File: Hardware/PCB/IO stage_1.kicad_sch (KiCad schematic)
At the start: 46 parts, among them IC10 THS4281DBVT, IC11 M74VHC1GT126DT1G, IC12 M74VHC1GT126DT1G, IC13 M74VHC1GT126DT1G, IC14 M74VHC1GT126DT1G, IC15 M74VHC1GT126DT1G, IC16 M74VHC1GT126DT1G, IC17 M74VHC1GT126DT1G, IC18 M74VHC1GT126DT1G, IC2 M74VHC1GT126DT1G, IC4 M74VHC1GT126DT1G, IC5 M74VHC1GT126DT1G, IC6 M74VHC1GT126DT1G, IC9 LP5907MFX-3.3, X10 conn 1x3, X2 conn 1x2, X4 conn 1x3, X5 conn 1x5, X8 CLCK_JACK, X9 conn 1x5

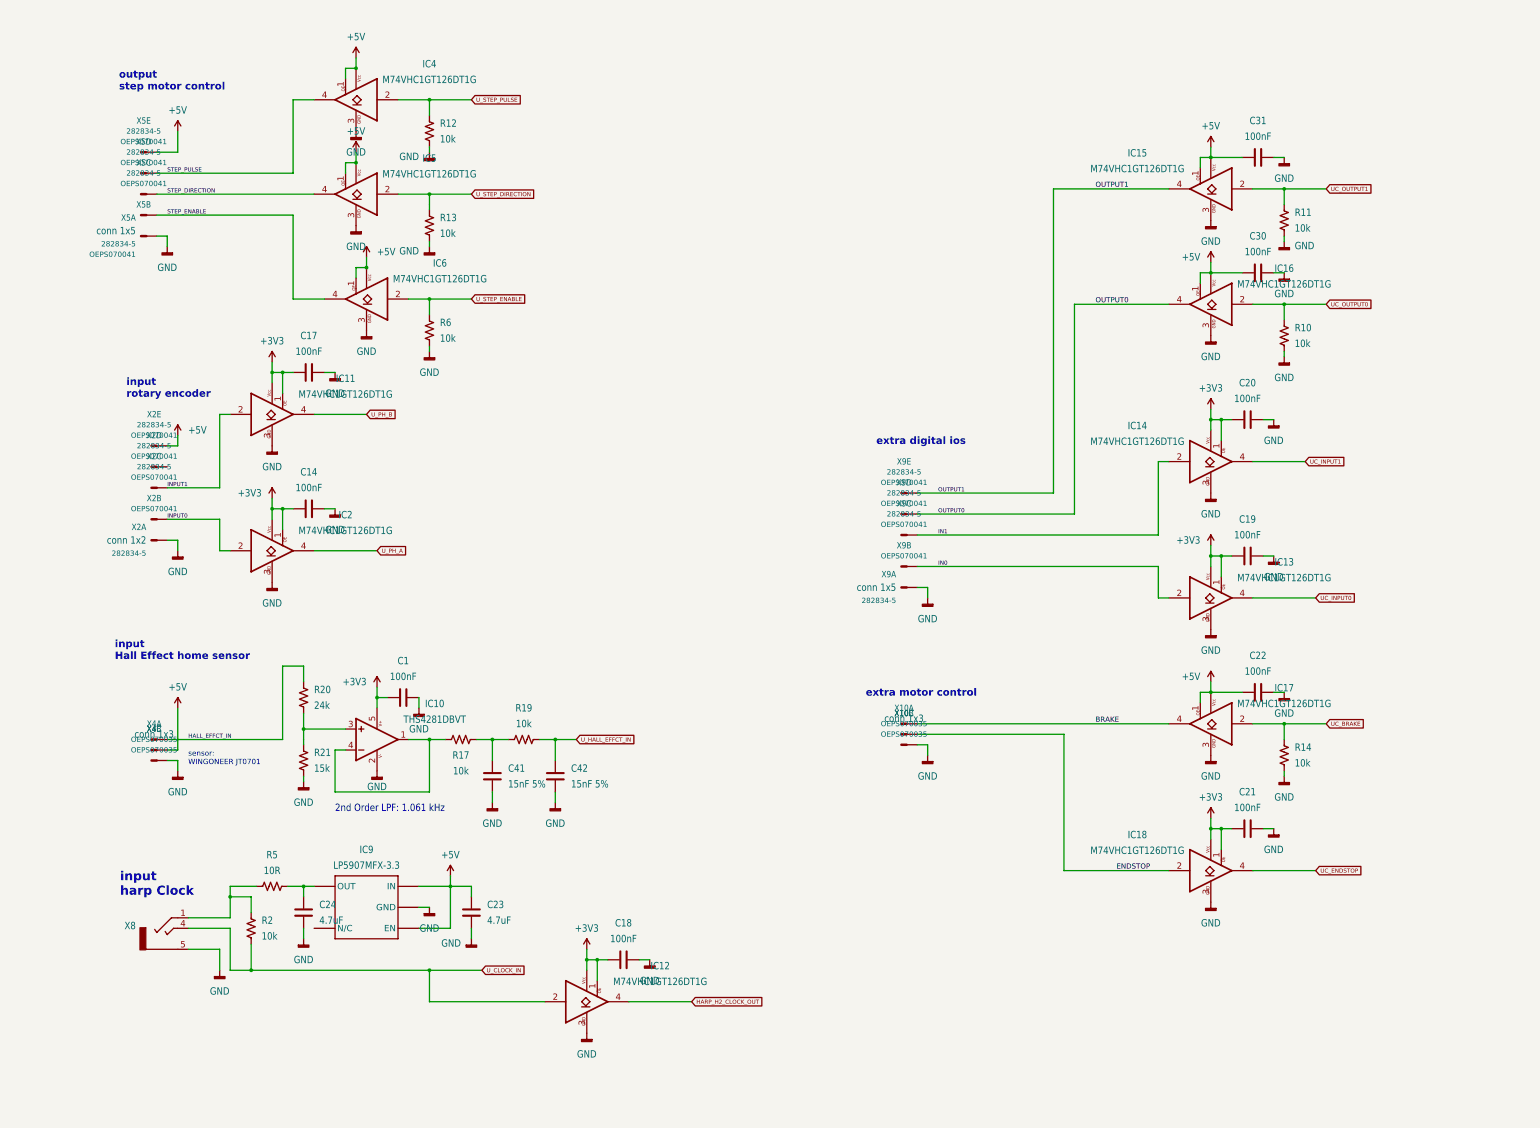
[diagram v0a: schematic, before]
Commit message: Implemented the new hardware features
Co-Authored-By: David Palma <78764277+davidpalma666@users.noreply.github.com>
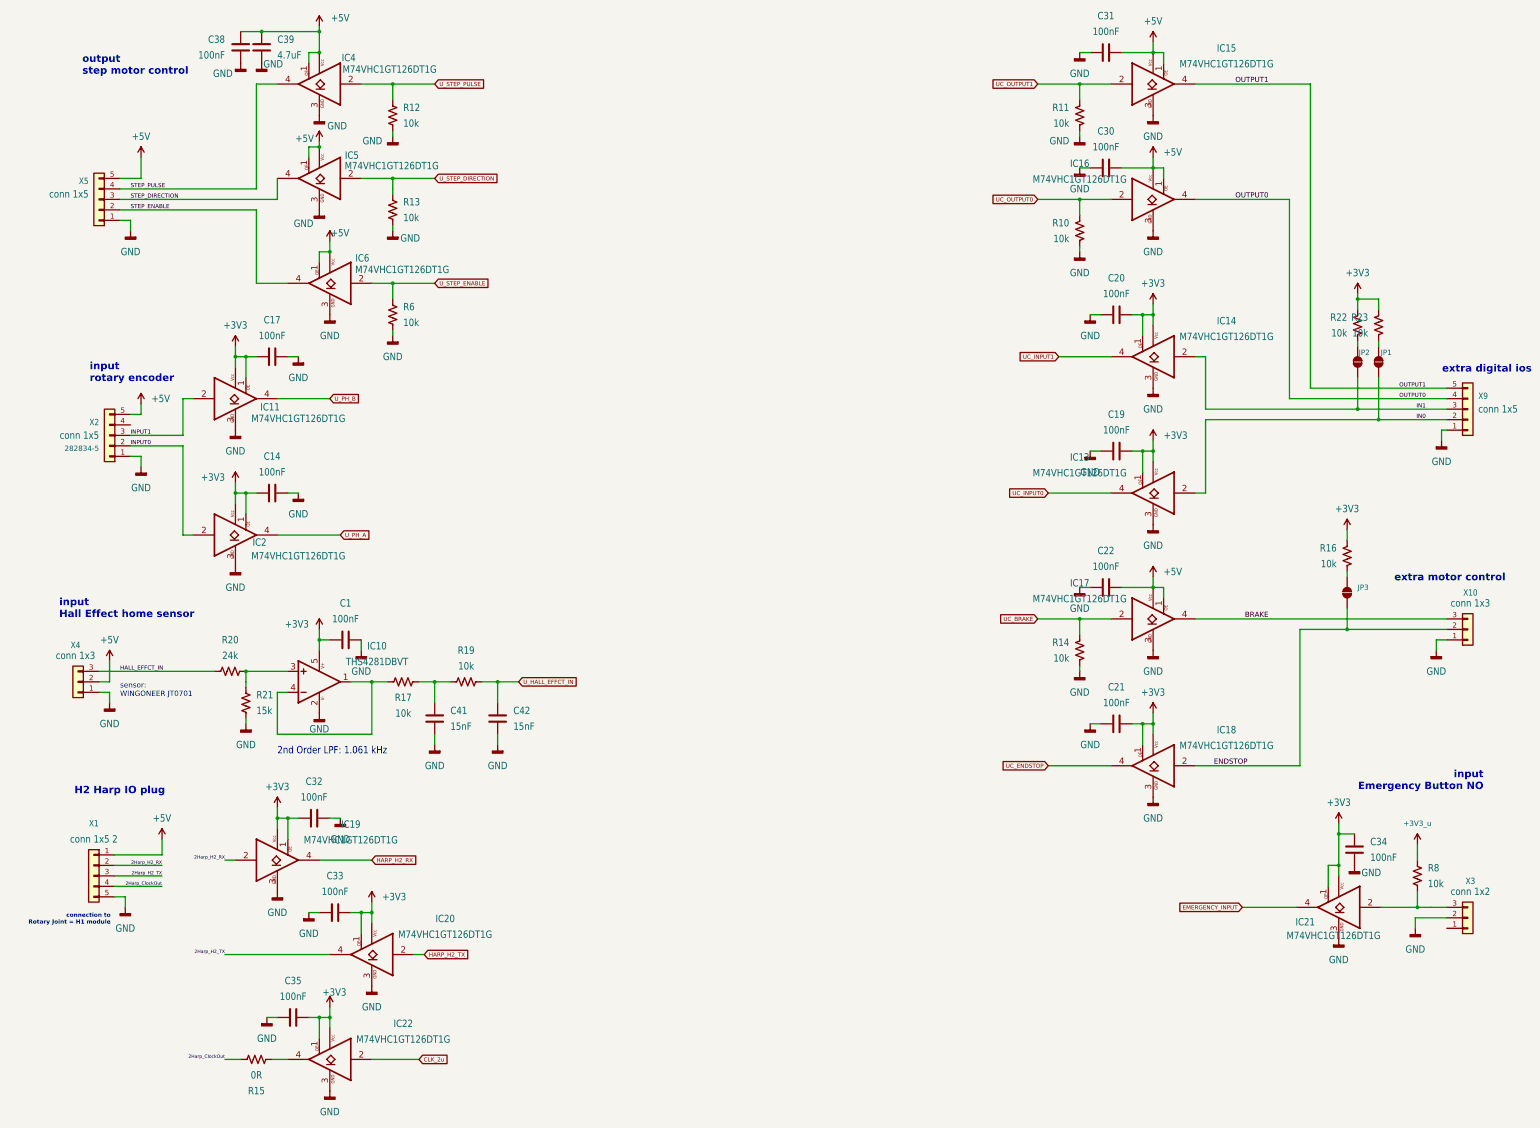
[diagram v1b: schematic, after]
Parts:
- removed C18: 100nF, FastStepper PCBLib:C0402K, symbol Device:C
- removed C23, C24: 4.7uF, FastStepper PCBLib:C0603K, symbol Device:C
- removed IC12: M74VHC1GT126DT1G, FastStepper PCBLib:TSOP-5, symbol FastStepper SymbLib:M74VHC1GT126DT1G
- removed IC9: LP5907MFX-3.3, FastStepper PCBLib:TSOT23-5, symbol FastStepper SymbLib:TLV700XX
- removed R2: 10k, FastStepper PCBLib:R0402, symbol Device:R_US
- removed R5: 10R, FastStepper PCBLib:R0402, symbol Device:R_US
- removed unit 2 of X10
- removed unit 3 of X10
- removed unit 4 of X2
- removed unit 5 of X2
- removed unit 2 of X2
- removed unit 3 of X2
- removed unit 2 of X4
- removed unit 3 of X4
- removed unit 2 of X5
- removed unit 3 of X5
- removed unit 4 of X5
- removed unit 5 of X5
- removed X8: CLCK_JACK, FastStepper PCBLib:35RASMT2BHNTRX, symbol FastStepper SymbLib:STEREO_JACK
- removed unit 2 of X9
- removed unit 3 of X9
- removed unit 5 of X9
- removed unit 4 of X9
- added C32, C33, C34, C35, C38: 100nF, Capacitor_SMD:C_0402_1005Metric, symbol Device:C
- added C39: 4.7uF, Capacitor_SMD:C_0603_1608Metric, symbol Device:C
- added IC19, IC20, IC21, IC22: M74VHC1GT126DT1G, Package_SO:TSOP-5_1.65x3.05mm_P0.95mm, symbol FastStepper SymbLib:M74VHC1GT126DT1G
- added JP1, JP2, JP3: SolderJumper_2_Open, Jumper:SolderJumper-2_P1.3mm_Open_RoundedPad1.0x1.5mm, symbol Jumper:SolderJumper_2_Open
- added R15: 0R, Resistor_SMD:R_0402_1005Metric, symbol Device:R_US
- added R16, R22, R23, R8: 10k, Resistor_SMD:R_0402_1005Metric, symbol Device:R_US
- added X1: conn 1x5 2, FastStepper PCBLib:90G-5, symbol Connector_Generic:Conn_01x05
- added X3: conn 1x2, FastStepper PCBLib:22-23-2031, symbol Connector_Generic:Conn_01x03
- C1, C14, C17, C19, C20, C21, C22, C30, C31: footprint FastStepper PCBLib:C0402K -> Capacitor_SMD:C_0402_1005Metric; MPN C1005X7R1H104K050BB -> CGA2B3X7R1H104K050BB; OEPS OEPS010004 -> (none); OEPSPN (none) -> OEPS010016
- C41, C42: value 15nF 5% -> 15nF; footprint FastStepper PCBLib:C0402K -> Capacitor_SMD:C_0402_1005Metric; OEPS OEPS010023 -> (none); OEPSPN (none) -> OEPS010023
- IC10: footprint FastStepper PCBLib:SOT23-5 -> Package_TO_SOT_SMD:SOT-23-5; OEPS OEPS080038 -> (none); OEPSPN (none) -> OEPS080038
- IC11, IC13, IC14, IC15, IC16, IC17, IC18, IC2, IC4, IC5, IC6: footprint FastStepper PCBLib:TSOP-5 -> Package_SO:TSOP-5_1.65x3.05mm_P0.95mm; DIGIKEY_PN M74VHC1GT126DT1GOSDKR-ND -> (none); OEPS OEPS080017 -> (none); OEPSPN (none) -> OEPS080017
- R10, R11, R12, R13, R14, R17, R19, R6: footprint FastStepper PCBLib:R0402 -> Resistor_SMD:R_0402_1005Metric; MPN CRCW040210K0FKED -> ERJ-2RKF1002X; OEPS OEPS020030 -> (none); OEPSPN (none) -> OEPS020013
- R20: footprint FastStepper PCBLib:R0402 -> Resistor_SMD:R_0402_1005Metric; OEPS OEPS020048 -> (none); OEPSPN (none) -> OEPS020048
- R21: footprint FastStepper PCBLib:R0402 -> Resistor_SMD:R_0402_1005Metric; OEPS OEPS020015 -> (none); OEPSPN (none) -> OEPS020015
- X10, X4: symbol FastStepper SymbLib:22-23-2031 -> Connector_Generic:Conn_01x03; OEPS OEPS070035 -> (none); OEPSPN (none) -> OEPS070035
- X2: value conn 1x2 -> conn 1x5; symbol FastStepper SymbLib:22-23-2051 -> Connector_Generic:Conn_01x05; OEPS OEPS070041 -> (none); OEPSPN (none) -> OEPS070041
- X5, X9: symbol FastStepper SymbLib:22-23-2051 -> Connector_Generic:Conn_01x05; OEPS OEPS070041 -> (none); OEPSPN (none) -> OEPS070041
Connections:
- net +3V3: now also C32.1, C33.1, C34.1, C35.1, IC19.1 (OE), IC19.5 (VCC), IC20.1 (OE), IC20.5 (VCC), IC21.1 (OE), IC21.5 (VCC), IC22.1 (OE), IC22.5 (VCC), R16.2, R22.2, R23.2
- net +5V: now also X2.5 (Pin_5), X4.2 (Pin_2), X5.5 (Pin_5), C38.2, C39.1, X1.1 (Pin_1)
- net BRAKE: now also X10.3 (Pin_3)
- net ENDSTOP: now also X10.2 (Pin_2), JP3.1 (A)
- net GND: now also C32.2, C33.2, C34.2, C35.2, C38.1, C39.2, IC19.3 (GND), IC20.3 (GND), IC21.3 (GND), IC22.3 (GND), X1.5 (Pin_5), X3.2 (Pin_2)
- net HALL_EFFCT_IN: now also X4.3 (Pin_3)
- net IN0: now also X9.2 (Pin_2), JP1.1 (A)
- net IN1: now also X9.3 (Pin_3), JP2.1 (A)
- net INPUT0: now also X2.2 (Pin_2)
- net INPUT1: now also X2.3 (Pin_3)
- net OUTPUT0: now also X9.4 (Pin_4)
- net OUTPUT1: now also X9.5 (Pin_5)
- net STEP_DIRECTION: now also X5.3 (Pin_3)
- net STEP_ENABLE: now also X5.2 (Pin_2)
- net STEP_PULSE: now also X5.4 (Pin_4)
- new net: JP3.2 (B), R16.1
- new net: IC21.2 (A), R8.1, X3.3 (Pin_3)
- new net: IC22.4 (Y), R15.1
- new net: JP1.2 (B), R23.1
- new net: JP2.2 (B), R22.1
- new net +3V3_u: R8.2
- new net 2Harp_ClockOut: R15.2, X1.4 (Pin_4)
- new net 2Harp_H2_RX: IC19.2 (A), X1.2 (Pin_2)
- new net 2Harp_H2_TX: IC20.4 (Y), X1.3 (Pin_3)
- new net CLK_2u: IC22.2 (A)
- new net EMERGENCY_INPUT: IC21.4 (Y)
- new net HARP_H2_RX: IC19.4 (Y)
- new net HARP_H2_TX: IC20.2 (A)
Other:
- note added: "H2 Harp IO plug"
- note added: "connection to Rotary Joint = H1 module"
- note added: "input Emergency Button NO"
- note removed: "input harp Clock"
- moved on the sheet: C1, C14, C17, C19, C20, C21, C22, C30, C31, C41, C42, IC10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
